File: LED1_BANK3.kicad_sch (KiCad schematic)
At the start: 76 parts, among them U17 STP16CPC26T

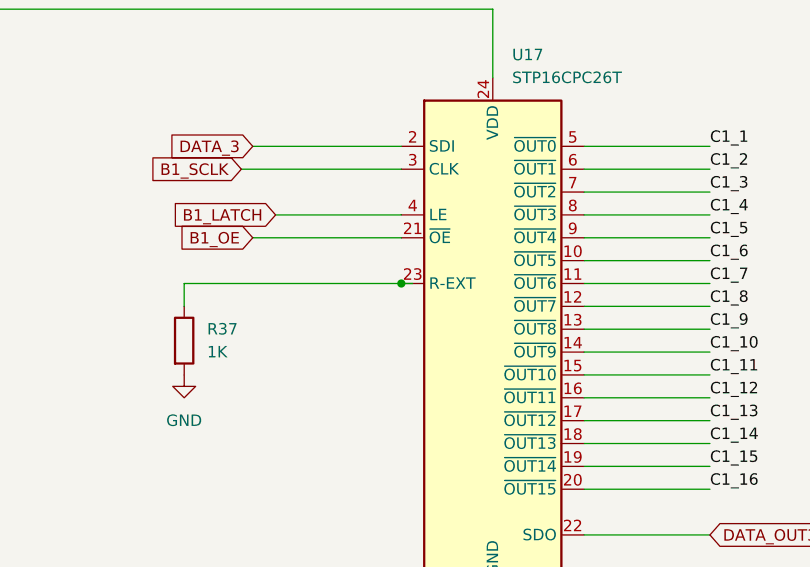
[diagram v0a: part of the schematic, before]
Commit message: sample
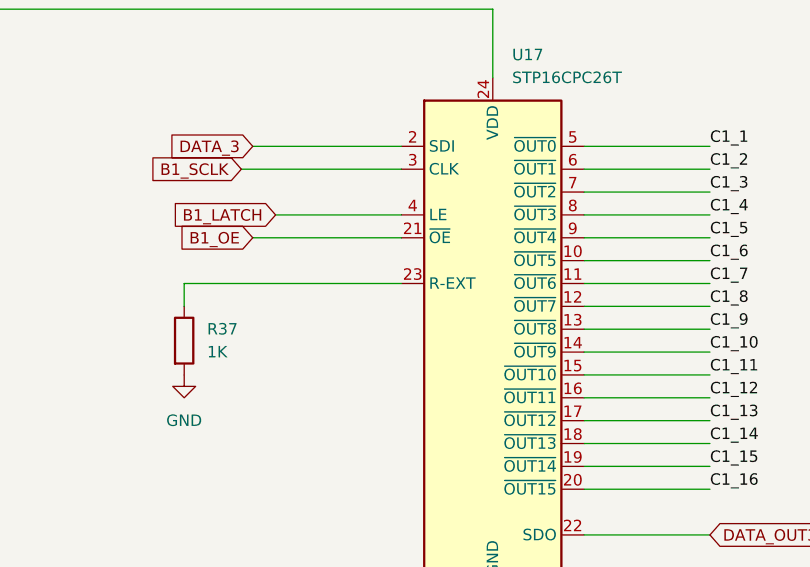
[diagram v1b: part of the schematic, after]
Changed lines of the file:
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@@
-	)
-	(junction
-		(at 86.36 160.02)
-		(diameter 0)
-		(color 0 0 0 0)
 	)
 	(junction
@@
 		)
 		(stroke
-			(width 0)
-			(type default)
-		)
-	)
-	(wire
-		(pts
-			(xy 86.36 160.02) (xy 87.63 160.02)
-		)
-		(stroke
